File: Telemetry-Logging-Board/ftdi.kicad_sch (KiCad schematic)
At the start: 14 parts, among them J8 USB_C_Receptacle_USB2.0_16P, U10 FT230XQ

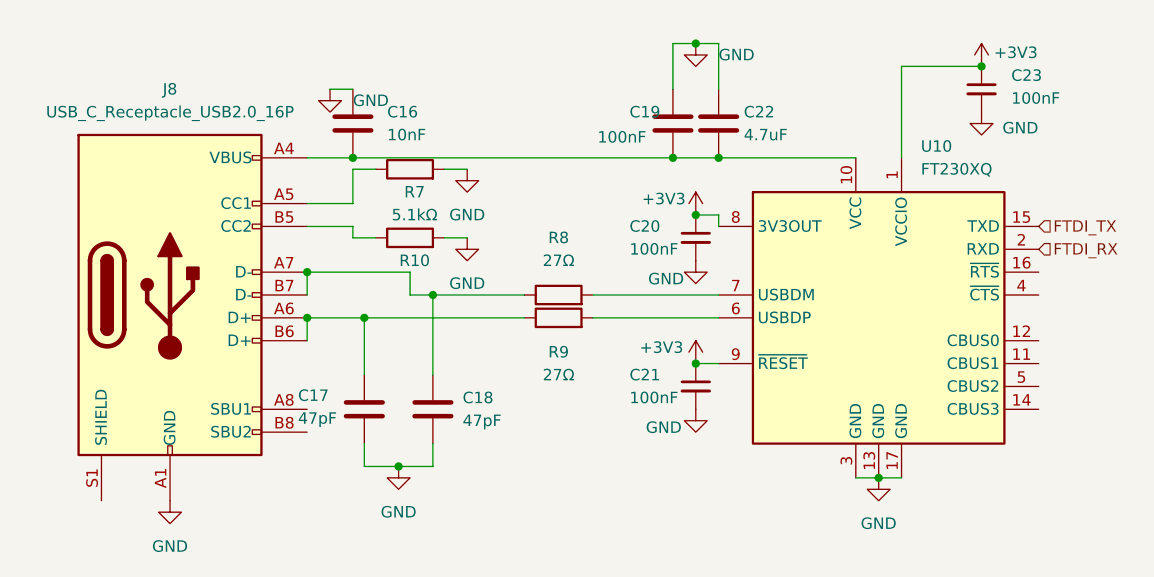
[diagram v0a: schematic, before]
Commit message: Change to same m.2 footprint as teledatics, fix some crystals, mess with layout
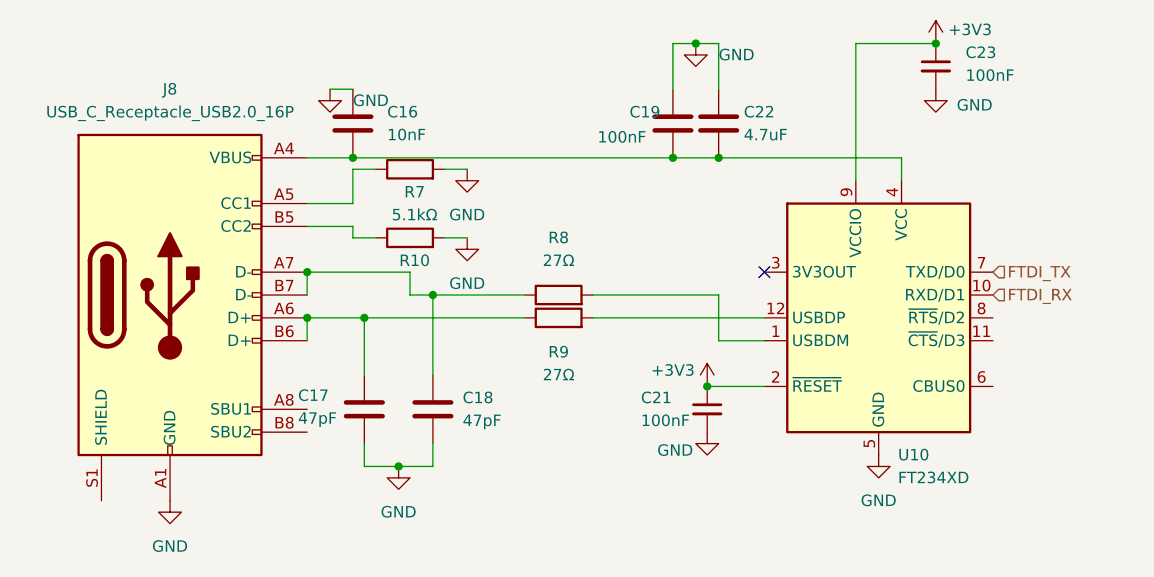
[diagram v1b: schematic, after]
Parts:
- removed C20: 100nF, Capacitor_SMD:C_0805_2012Metric_Pad1.18x1.45mm_HandSolder, symbol Device:C_Small
- removed U10: FT230XQ, Package_DFN_QFN:QFN-16-1EP_4x4mm_P0.65mm_EP2.1x2.1mm, symbol Interface_USB:FT230XQ
- added U10: FT234XD, Package_DFN_QFN:WDFN-12-1EP_3x3mm_P0.45mm_EP1.7x2.5mm, symbol Interface_USB:FT234XD
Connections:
- net +3V3: now also U10.2 (~{RESET}), U10.9 (VCCIO)
- net FTDI_RX: now also U10.10 (RXD/D1)
- net FTDI_TX: now also U10.7 (TXD/D0)
- net GND: now also U10.13 (GND), U10.5 (GND)
- net at R9.2: now also U10.12 (USBDP)
- net at C16.2, C19.2, C22.2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: now also U10.4 (VCC)
- net at R8.2: now also U10.1 (USBDM)
- no-connect marks 0 -> 1
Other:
- moved on the sheet: C21, C23
